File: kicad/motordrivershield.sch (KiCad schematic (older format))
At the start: 51 parts, among them CN1 ARDUINO_MKR, CN2 QWIIC, CN3 ARDUINO_NANO_33, P1 CONN_01X03, P2 CONN_01X03, U1 PCA9685_TSSOP28, U2 ADS1015

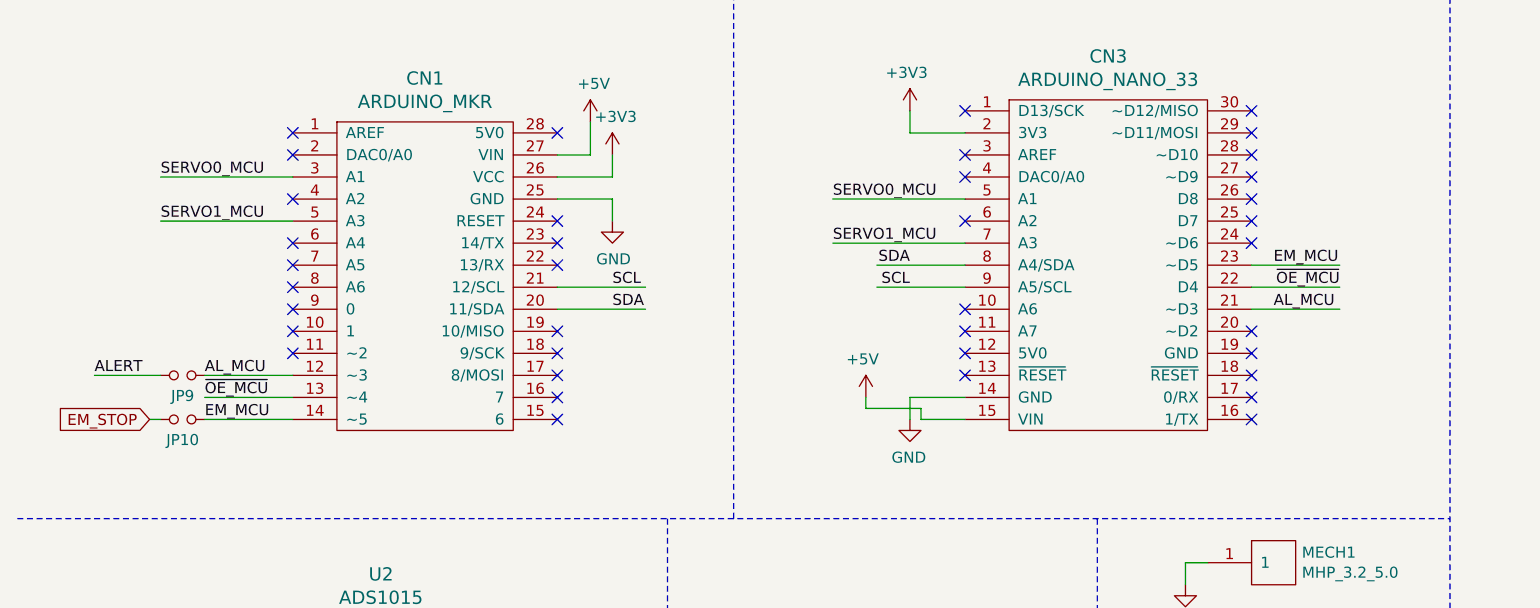
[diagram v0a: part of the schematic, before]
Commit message: servos angepasst
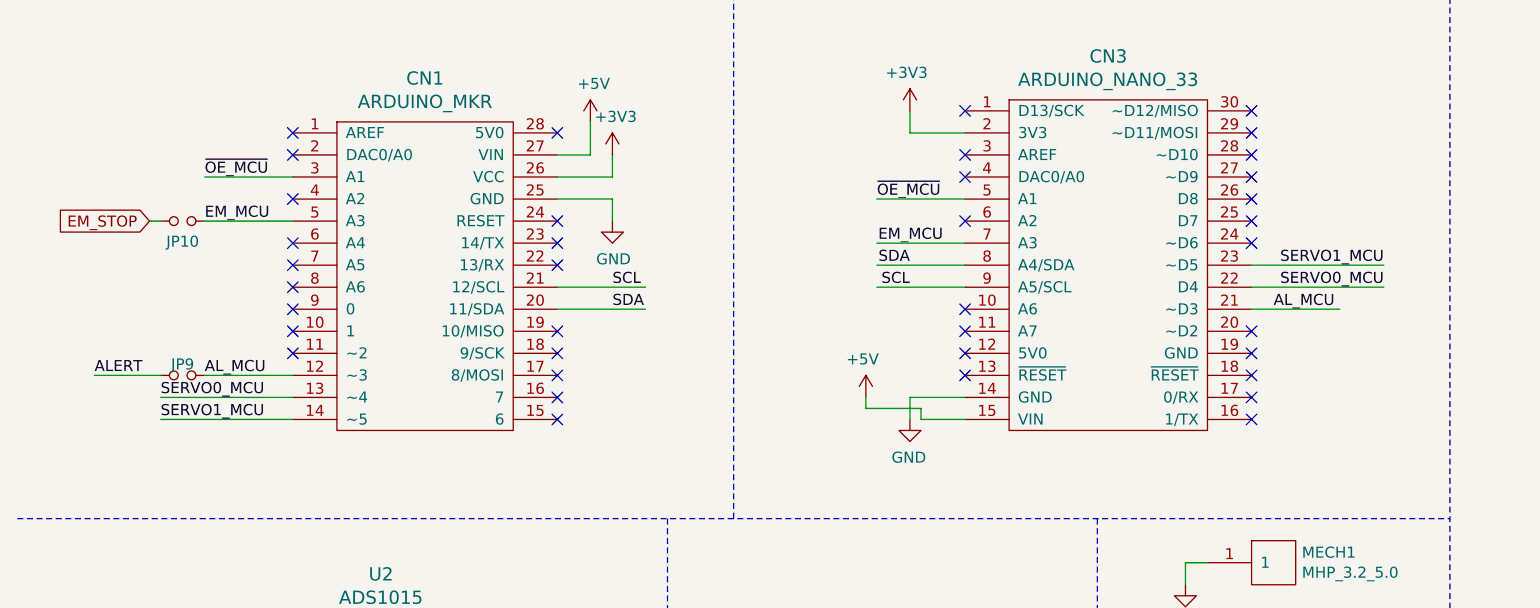
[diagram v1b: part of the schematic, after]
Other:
- moved on the sheet: JP10
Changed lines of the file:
@@
 $EndComp
 Wire Wire Line
-	1750 2400 1350 2400
-Wire Wire Line
-	1750 2500 1350 2500
+	1750 1400 1350 1400
+Wire Wire Line
+	1750 1600 1350 1600
 Wire Wire Line
 	2950 2000 3350 2000
 Wire Wire Line
 	2950 1900 3350 1900
-Text Label 1350 2400 0    50   ~ 0
+Text Label 1350 1400 0    50   ~ 0
 ~OE_MCU
-Text GLabel 1100 2500 0    50   Input ~ 0
+Text GLabel 1100 1600 0    50   Input ~ 0
 EM_STOP
 Text Label 3200 1900 0    50   ~ 0
@@
 U 1 1 5F60D737
 P 1250 2300
-F 0 "JP9" H 1250 2393 50  0000 C CNN
+F 0 "JP9" H 1250 2250 50  0000 C CNN
 F 1 "Jumper_NO_Small" H 1260 2240 50  0001 C CNN
 F 2 "wire_pads:SolderJumper_2mm" H 1250 2250 50  0001 C CNN
@@
 L devices:Jumper_NO_Small JP10
 U 1 1 5F61363A
-P 1250 2500
-F 0 "JP10" H 1250 2593 50  0000 C CNN
-F 1 "Jumper_NO_Small" H 1260 2440 50  0001 C CNN
-F 2 "wire_pads:SolderJumper_2mm" H 1250 2450 50  0001 C CNN
-F 3 "" H 1250 2500 50  0000 C CNN
-	1    1250 2500
+P 1250 1600
+F 0 "JP10" H 1250 1693 50  0000 C CNN
+F 1 "Jumper_NO_Small" H 1260 1540 50  0001 C CNN
+F 2 "wire_pads:SolderJumper_2mm" H 1250 1550 50  0001 C CNN
+F 3 "" H 1250 1600 50  0000 C CNN
+	1    1250 1600
 	-1   0    0    1
 $EndComp
@@
 	1150 2300 850  2300
 Wire Wire Line
-	1150 2500 1100 2500
+	1150 1600 1100 1600
 Wire Wire Line
 	2950 1300 3100 1300
@@
 SDA
 Wire Wire Line
-	6100 1900 6500 1900
+	4800 1500 4400 1500
 Wire Wire Line
 	6100 2000 6500 2000
-Text Label 6500 1900 2    50   ~ 0
+Text Label 4400 1500 0    50   ~ 0
 ~OE_MCU
 Wire Wire Line
-	6100 1800 6500 1800
+	4800 1700 4400 1700
 Text Label 1350 2300 0    50   ~ 0
 AL_MCU
-Text Label 1350 2500 0    50   ~ 0
+Text Label 1350 1600 0    50   ~ 0
 EM_MCU
 Text Label 6200 2000 0    50   ~ 0
 AL_MCU
-Text Label 6200 1800 0    50   ~ 0
+Text Label 4700 1700 2    50   ~ 0
 EM_MCU
 NoConn ~ 6100 1100
@@
 Text Label 10250 1950 0    50   ~ 0
 SERVO1_PCA
-Text Label 4200 1500 0    50   ~ 0
+Text Label 6700 1900 2    50   ~ 0
 SERVO0_MCU
 Wire Wire Line
-	4200 1500 4800 1500
-Wire Wire Line
-	4200 1700 4800 1700
-Text Label 4200 1700 0    50   ~ 0
+	6700 1900 6100 1900
+Wire Wire Line
+	6700 1800 6100 1800
+Text Label 6700 1800 2    50   ~ 0
 SERVO1_MCU
-Text Label 1150 1400 0    50   ~ 0
+Text Label 1150 2400 0    50   ~ 0
 SERVO0_MCU
 Wire Wire Line
-	1150 1400 1750 1400
-Wire Wire Line
-	1150 1600 1750 1600
-Text Label 1150 1600 0    50   ~ 0
+	1150 2400 1750 2400
+Wire Wire Line
+	1150 2500 1750 2500
+Text Label 1150 2500 0    50   ~ 0
 SERVO1_MCU
 $Comp

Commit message: blöder servo
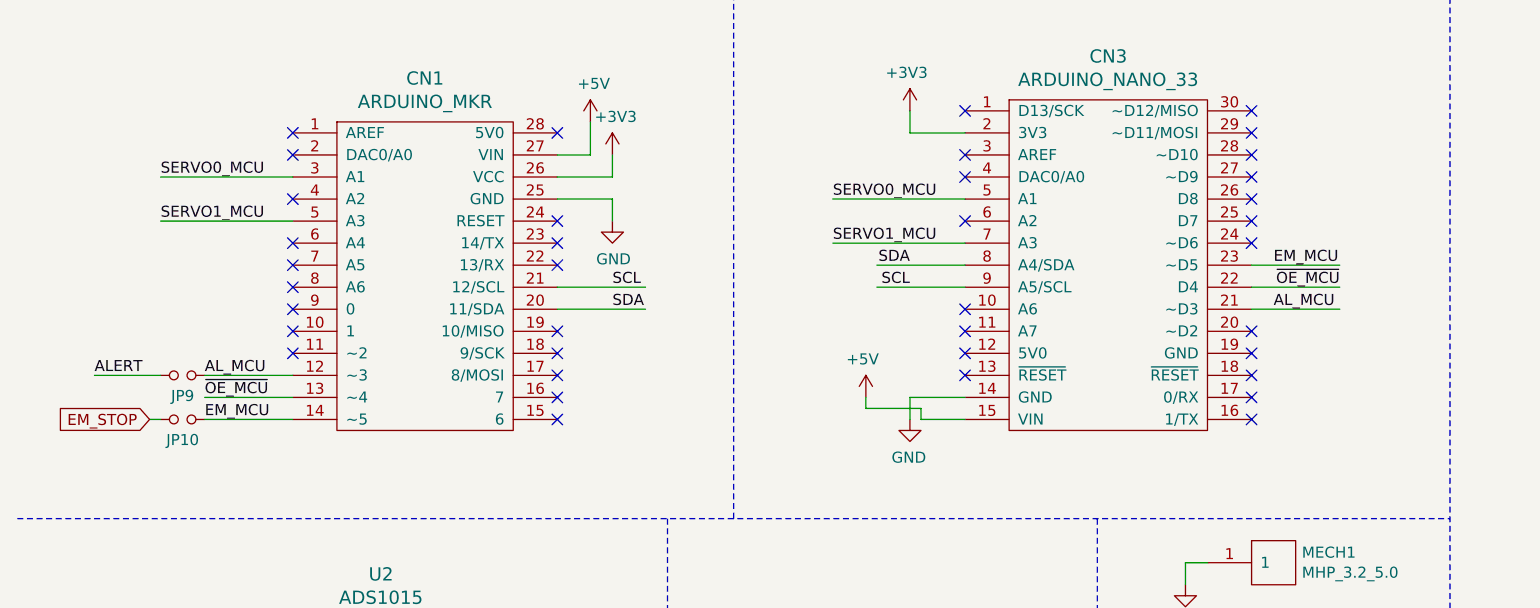
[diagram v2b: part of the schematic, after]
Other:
- moved on the sheet: JP10
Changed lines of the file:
@@
 $EndComp
 Wire Wire Line
-	1750 1400 1350 1400
-Wire Wire Line
-	1750 1600 1350 1600
+	1750 2400 1350 2400
+Wire Wire Line
+	1750 2500 1350 2500
 Wire Wire Line
 	2950 2000 3350 2000
 Wire Wire Line
 	2950 1900 3350 1900
-Text Label 1350 1400 0    50   ~ 0
+Text Label 1350 2400 0    50   ~ 0
 ~OE_MCU
-Text GLabel 1100 1600 0    50   Input ~ 0
+Text GLabel 1100 2500 0    50   Input ~ 0
 EM_STOP
 Text Label 3200 1900 0    50   ~ 0
@@
 U 1 1 5F60D737
 P 1250 2300
-F 0 "JP9" H 1250 2250 50  0000 C CNN
+F 0 "JP9" H 1250 2393 50  0000 C CNN
 F 1 "Jumper_NO_Small" H 1260 2240 50  0001 C CNN
 F 2 "wire_pads:SolderJumper_2mm" H 1250 2250 50  0001 C CNN
@@
 L devices:Jumper_NO_Small JP10
 U 1 1 5F61363A
-P 1250 1600
-F 0 "JP10" H 1250 1693 50  0000 C CNN
-F 1 "Jumper_NO_Small" H 1260 1540 50  0001 C CNN
-F 2 "wire_pads:SolderJumper_2mm" H 1250 1550 50  0001 C CNN
-F 3 "" H 1250 1600 50  0000 C CNN
-	1    1250 1600
+P 1250 2500
+F 0 "JP10" H 1250 2593 50  0000 C CNN
+F 1 "Jumper_NO_Small" H 1260 2440 50  0001 C CNN
+F 2 "wire_pads:SolderJumper_2mm" H 1250 2450 50  0001 C CNN
+F 3 "" H 1250 2500 50  0000 C CNN
+	1    1250 2500
 	-1   0    0    1
 $EndComp
@@
 	1150 2300 850  2300
 Wire Wire Line
-	1150 1600 1100 1600
+	1150 2500 1100 2500
 Wire Wire Line
 	2950 1300 3100 1300
@@
 SDA
 Wire Wire Line
-	4800 1500 4400 1500
+	6100 1900 6500 1900
 Wire Wire Line
 	6100 2000 6500 2000
-Text Label 4400 1500 0    50   ~ 0
+Text Label 6500 1900 2    50   ~ 0
 ~OE_MCU
 Wire Wire Line
-	4800 1700 4400 1700
+	6100 1800 6500 1800
 Text Label 1350 2300 0    50   ~ 0
 AL_MCU
-Text Label 1350 1600 0    50   ~ 0
+Text Label 1350 2500 0    50   ~ 0
 EM_MCU
 Text Label 6200 2000 0    50   ~ 0
 AL_MCU
-Text Label 4700 1700 2    50   ~ 0
+Text Label 6200 1800 0    50   ~ 0
 EM_MCU
 NoConn ~ 6100 1100
@@
 Text Label 10250 1950 0    50   ~ 0
 SERVO1_PCA
-Text Label 6700 1900 2    50   ~ 0
+Text Label 4200 1500 0    50   ~ 0
 SERVO0_MCU
 Wire Wire Line
-	6700 1900 6100 1900
-Wire Wire Line
-	6700 1800 6100 1800
-Text Label 6700 1800 2    50   ~ 0
+	4200 1500 4800 1500
+Wire Wire Line
+	4200 1700 4800 1700
+Text Label 4200 1700 0    50   ~ 0
 SERVO1_MCU
-Text Label 1150 2400 0    50   ~ 0
+Text Label 1150 1400 0    50   ~ 0
 SERVO0_MCU
 Wire Wire Line
-	1150 2400 1750 2400
-Wire Wire Line
-	1150 2500 1750 2500
-Text Label 1150 2500 0    50   ~ 0
+	1150 1400 1750 1400
+Wire Wire Line
+	1150 1600 1750 1600
+Text Label 1150 1600 0    50   ~ 0
 SERVO1_MCU
 $Comp
